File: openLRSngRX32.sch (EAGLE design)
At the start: 58 parts, among them IC1 STM32F10XCXT6, IC2 REG1117, U1 MPU-6000QFN-24, Y1 8MHz

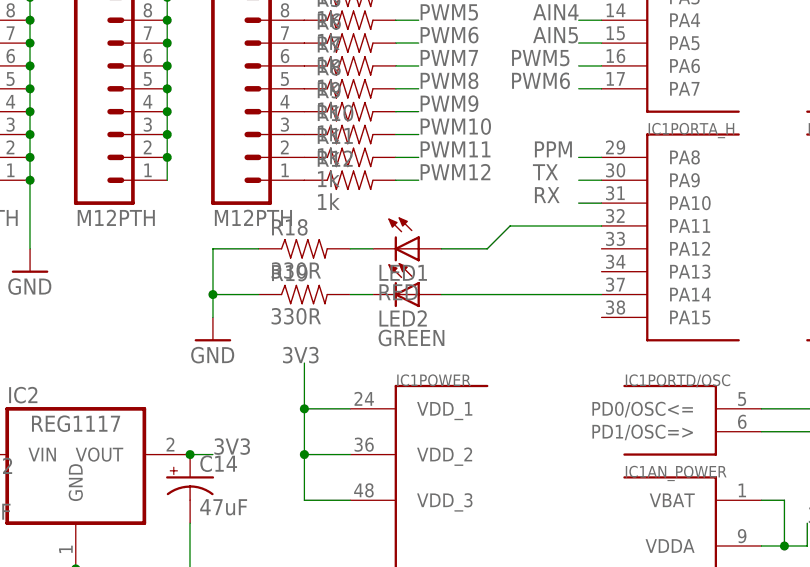
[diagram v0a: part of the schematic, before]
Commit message: GB leds
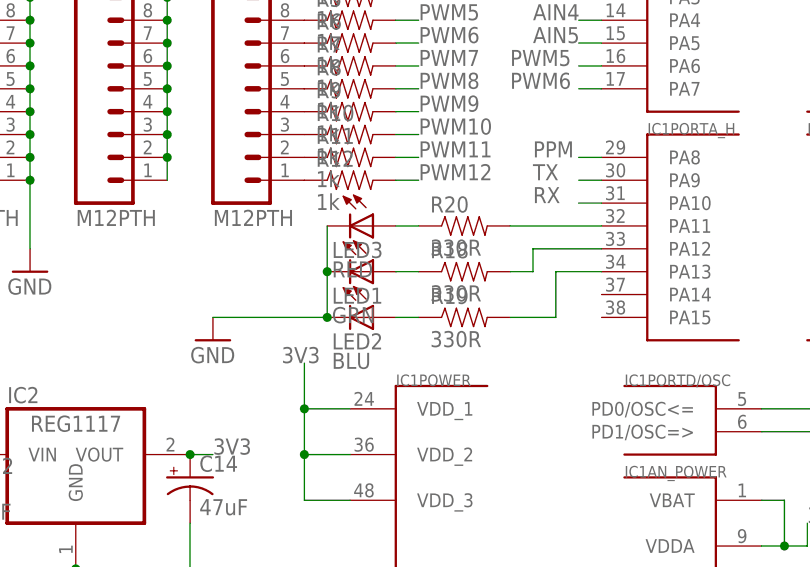
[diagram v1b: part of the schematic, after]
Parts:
- added LED3: RED, led:LEDSML0805
- added R20: 330R, SparkFun-Resistors:RESISTOR0805-RES
- LED1: value RED -> GRN
- LED2: value GREEN -> BLU
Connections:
- removed net N$29: LED1.C, R18.2
- new net N$33: IC1PORTA_H.PA11, R20.2
- new net N$34: IC1PORTA_H.PA12, R18.2
- new net N$35: IC1PORTA_H.PA13, R19.2
- net GND: now also LED1.C, LED2.C, LED3.C; no longer R18.1, R19.1
- net N$30: now also LED3.A, R20.1; no longer LED2.C, R19.2
- net N$31: now also R18.1; no longer IC1PORTA_H.PA11
- net N$32: now also R19.1; no longer IC1PORTA_H.PA14
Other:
- moved on the sheet: LED1, LED2, R18, R19
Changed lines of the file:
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@@
 <part name="JP11" library="SparkFun-Connectors" deviceset="M02" device="PTH"/>
 <part name="C17" library="SparkFun-Capacitors" deviceset="CAP" device="0805"/>
-<part name="LED1" library="led" deviceset="LED" device="SML0805" value="RED"/>
-<part name="LED2" library="led" deviceset="LED" device="SML0805" value="GREEN"/>
+<part name="LED1" library="led" deviceset="LED" device="SML0805" value="GRN"/>
+<part name="LED2" library="led" deviceset="LED" device="SML0805" value="BLU"/>
 <part name="R18" library="SparkFun-Resistors" deviceset="RESISTOR" device="0805-RES" value="330R"/>
 <part name="R19" library="SparkFun-Resistors" deviceset="RESISTOR" device="0805-RES" value="330R"/>
 <part name="GND18" library="supply1" deviceset="GND" device=""/>
+<part name="LED3" library="led" deviceset="LED" device="SML0805" value="RED"/>
+<part name="R20" library="SparkFun-Resistors" deviceset="RESISTOR" device="0805-RES" value="330R"/>
 </parts>
 <sheets>
@@
 <instance part="JP11" gate="G$1" x="-45.72" y="22.86"/>
 <instance part="C17" gate="G$1" x="-78.74" y="33.02"/>
-<instance part="LED1" gate="G$1" x="27.94" y="58.42" rot="R270"/>
-<instance part="LED2" gate="G$1" x="27.94" y="53.34" rot="R270"/>
-<instance part="R18" gate="G$1" x="15.24" y="58.42"/>
-<instance part="R19" gate="G$1" x="15.24" y="53.34"/>
+<instance part="LED1" gate="G$1" x="22.86" y="55.88" rot="R270"/>
+<instance part="LED2" gate="G$1" x="22.86" y="50.8" rot="R270"/>
+<instance part="R18" gate="G$1" x="33.02" y="55.88"/>
+<instance part="R19" gate="G$1" x="33.02" y="50.8"/>
 <instance part="GND18" gate="1" x="5.08" y="48.26"/>
+<instance part="LED3" gate="G$1" x="22.86" y="60.96" rot="R270"/>
+<instance part="R20" gate="G$1" x="33.02" y="60.96"/>
 </instances>
 <busses>
@@
 </segment>
 <segment>
+<pinref part="LED3" gate="G$1" pin="C"/>
+<pinref part="LED1" gate="G$1" pin="C"/>
+<wire x1="17.78" y1="60.96" x2="17.78" y2="55.88" width="0.1524" layer="91"/>
+<pinref part="LED2" gate="G$1" pin="C"/>
+<wire x1="17.78" y1="55.88" x2="17.78" y2="50.8" width="0.1524" layer="91"/>
 <pinref part="GND18" gate="1" pin="GND"/>
-<pinref part="R19" gate="G$1" pin="1"/>
-<wire x1="5.08" y1="50.8" x2="5.08" y2="53.34" width="0.1524" layer="91"/>
-<wire x1="5.08" y1="53.34" x2="10.16" y2="53.34" width="0.1524" layer="91"/>
-<pinref part="R18" gate="G$1" pin="1"/>
-<wire x1="5.08" y1="53.34" x2="5.08" y2="58.42" width="0.1524" layer="91"/>
-<wire x1="5.08" y1="58.42" x2="10.16" y2="58.42" width="0.1524" layer="91"/>
-<junction x="5.08" y="53.34"/>
+<wire x1="17.78" y1="50.8" x2="5.08" y2="50.8" width="0.1524" layer="91"/>
+<junction x="17.78" y="55.88"/>
+<junction x="17.78" y="50.8"/>
 </segment>
 </net>
@@
 </segment>
 </net>
-<net name="N$29" class="0">
-<segment>
-<pinref part="R18" gate="G$1" pin="2"/>
-<pinref part="LED1" gate="G$1" pin="C"/>
-<wire x1="20.32" y1="58.42" x2="22.86" y2="58.42" width="0.1524" layer="91"/>
-</segment>
-</net>
 <net name="N$30" class="0">
 <segment>
-<pinref part="R19" gate="G$1" pin="2"/>
-<pinref part="LED2" gate="G$1" pin="C"/>
-<wire x1="20.32" y1="53.34" x2="22.86" y2="53.34" width="0.1524" layer="91"/>
+<pinref part="LED3" gate="G$1" pin="A"/>
+<pinref part="R20" gate="G$1" pin="1"/>
+<wire x1="25.4" y1="60.96" x2="27.94" y2="60.96" width="0.1524" layer="91"/>
 </segment>
 </net>
@@
 <segment>
 <pinref part="LED1" gate="G$1" pin="A"/>
-<wire x1="30.48" y1="58.42" x2="35.56" y2="58.42" width="0.1524" layer="91"/>
-<wire x1="35.56" y1="58.42" x2="38.1" y2="60.96" width="0.1524" layer="91"/>
+<pinref part="R18" gate="G$1" pin="1"/>
+<wire x1="25.4" y1="55.88" x2="27.94" y2="55.88" width="0.1524" layer="91"/>
+</segment>
+</net>
+<net name="N$32" class="0">
+<segment>
+<pinref part="LED2" gate="G$1" pin="A"/>
+<pinref part="R19" gate="G$1" pin="1"/>
+<wire x1="25.4" y1="50.8" x2="27.94" y2="50.8" width="0.1524" layer="91"/>
+</segment>
+</net>
+<net name="N$33" class="0">
+<segment>
+<pinref part="R20" gate="G$1" pin="2"/>
 <pinref part="IC1" gate="PORTA_H" pin="PA11"/>
 <wire x1="38.1" y1="60.96" x2="48.26" y2="60.96" width="0.1524" layer="91"/>
 </segment>
 </net>
-<net name="N$32" class="0">
-<segment>
-<pinref part="LED2" gate="G$1" pin="A"/>
-<pinref part="IC1" gate="PORTA_H" pin="PA14"/>
-<wire x1="30.48" y1="53.34" x2="48.26" y2="53.34" width="0.1524" layer="91"/>
-</segment>
-</net>
+<net name="N$34" class="0">
+<segment>
+<pinref part="R18" gate="G$1" pin="2"/>
+<wire x1="38.1" y1="55.88" x2="40.64" y2="55.88" width="0.1524" layer="91"/>
+<wire x1="40.64" y1="55.88" x2="40.64" y2="58.42" width="0.1524" layer="91"/>
+<pinref part="IC1" gate="PORTA_H" pin="PA12"/>
+<wire x1="40.64" y1="58.42" x2="48.26" y2="58.42" width="0.1524" layer="91"/>
+</segment>
+</net>
+<net name="N$35" class="0">
+<segment>
+<pinref part="R19" gate="G$1" pin="2"/>
+<wire x1="38.1" y1="50.8" x2="43.18" y2="50.8" width="0.1524" layer="91"/>
+<wire x1="43.18" y1="50.8" x2="43.18" y2="55.88" width="0.1524" layer="91"/>
+<pinref part="IC1" gate="PORTA_H" pin="PA13"/>
+<wire x1="43.18" y1="55.88" x2="48.26" y2="55.88" width="0.1524" layer="91"/>
+</segment>
+</net>
